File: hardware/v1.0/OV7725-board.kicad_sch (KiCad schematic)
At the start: 21 parts, among them J11 Conn_01x04, J12 Conn_01x34, J13 Conn_02x10_Odd_Even, U11 TLV62585, Y2 TFOM24M4RHKCNT2T

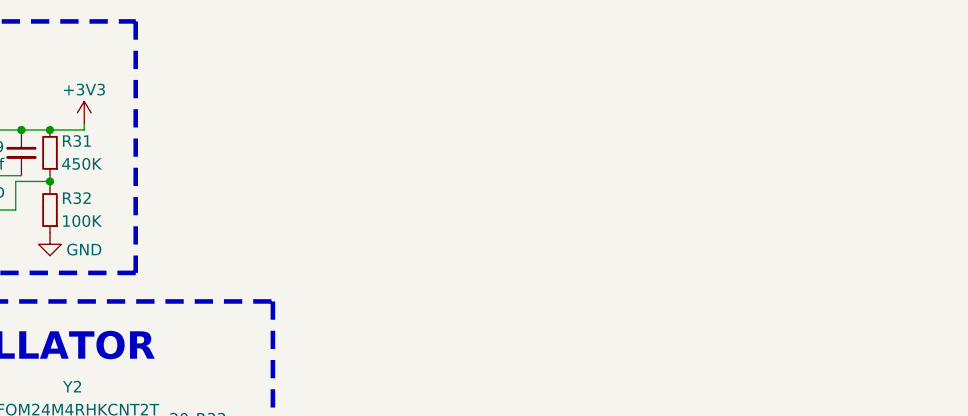
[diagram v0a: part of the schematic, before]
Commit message: changes
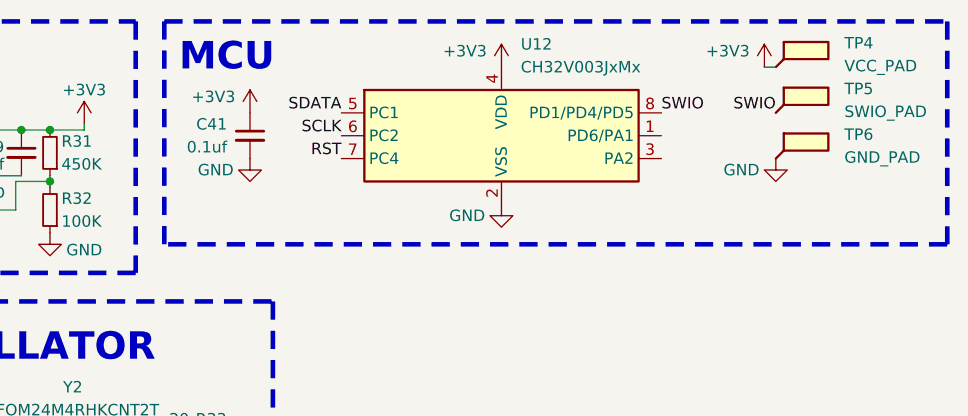
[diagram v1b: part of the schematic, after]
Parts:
- added C41: 0.1uf, Capacitor_SMD:C_0603_1608Metric, symbol Device:C_Small
- added TP4: VCC_PAD, TestPoint:TestPoint_Pad_D1.5mm, symbol Connector:TestPoint_Flag
- added TP5: SWIO_PAD, TestPoint:TestPoint_Pad_D1.5mm, symbol Connector:TestPoint_Flag
- added TP6: GND_PAD, TestPoint:TestPoint_Pad_D1.5mm, symbol Connector:TestPoint_Flag
- added U12: CH32V003JxMx, Package_SO:SOP-8_3.9x4.9mm_P1.27mm, symbol MCU_WCH_CH32V0:CH32V003JxMx
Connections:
- net +3V3: now also C41.1, TP4.1, U12.4 (VDD)
- net GND: now also C41.2, TP6.1, U12.2 (VSS)
- net RST: now also U12.7 (PC4)
- net SCLK: now also U12.6 (PC2)
- net SDATA: now also U12.5 (PC1)
- new net SWIO: TP5.1, U12.8 (PD1/PD4/PD5)
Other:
- note added: "MCU"

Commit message: changes
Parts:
- R31, R32: footprint Resistor_SMD:R_0402_1005Metric -> Resistor_SMD:R_0603_1608Metric
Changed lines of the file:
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@@
 			)
 		)
-		(property "Footprint" "Resistor_SMD:R_0402_1005Metric"
+		(property "Footprint" "Resistor_SMD:R_0603_1608Metric"
 			(at 141.605 34.925 0)
 			(effects
@@
 			)
 		)
-		(property "Footprint" "Resistor_SMD:R_0402_1005Metric"
+		(property "Footprint" "Resistor_SMD:R_0603_1608Metric"
 			(at 141.605 28.575 0)
 			(effects
